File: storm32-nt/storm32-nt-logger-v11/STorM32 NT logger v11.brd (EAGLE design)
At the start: 15.5 x 20 mm, 22 parts, among them IC1 STM32F10XTXU6, IC3 MPU9250, Q1 RESONATORSMD

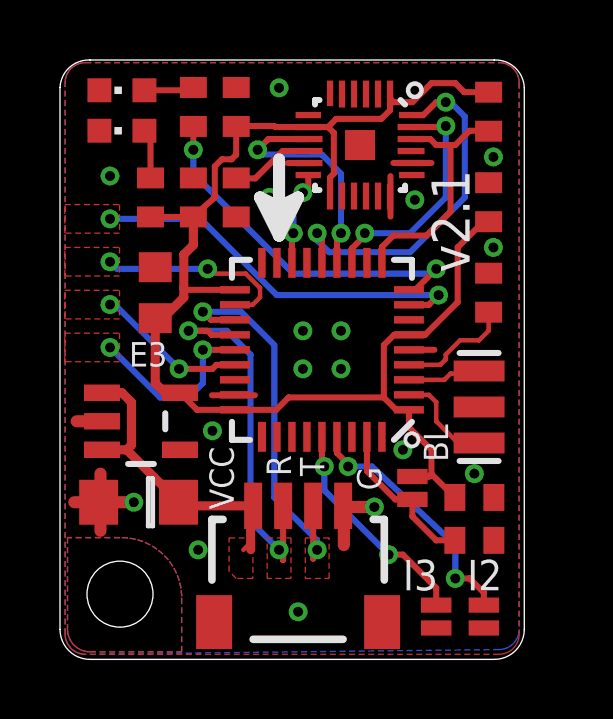
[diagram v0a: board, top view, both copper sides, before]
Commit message: release board v3.3, motor v2.5E, oled, esp
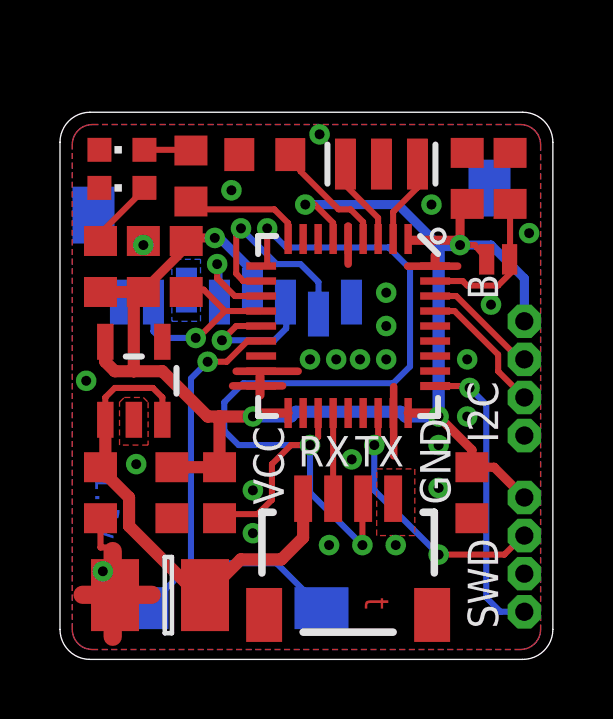
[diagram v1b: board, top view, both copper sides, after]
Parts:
- removed C3, C4, C5, C6: 100n, rcl:C0402
- removed IC1: STM32F10XTXU6, # stm32:VFQFPN36
- removed IC3: MPU9250, # SparkFun2:QFN-24-3X3
- removed NT: NT, con-jst2:SM04B-SRSS-TB
- removed Q1: RESONATORSMD, # SparkFun2:RESONATOR-SMD
- removed R5: 10k, rcl:R0402
- removed SJ1: BOOT0, # SparkFun2:SJ_2S-NO
- removed SJ3: IMU-ID3, # SparkFun2:SJ_2S-NO
- added C10, C11, C9: 100n, rcl:C0603
- added JP1, JP2: SWD, # stdlib:4X1_1P27_OCT_BILEX
- added NTX: NTX, con-jst2:SM04B-SRSS-TB
- added R6: 2.2k, rcl:R0603
- added R7: 10k, rcl:R0603
- added U$1: MICROSD, # adafruit:MICROSD
- added U1: STM32F10XTXU6, # stm32:VFQFPN36
- added Y1: RESONATORSMD, # SparkFun2:RESONATOR-SMD
- C1: device rcl:C0805 -> rcl:SMC_B
- C2: value 1u -> 100n
- C7: value 10n -> 1u; device rcl:C0402 -> rcl:C0603
- C8: device rcl:C0402 -> rcl:C0603
- R1: value 10k -> 4.7k; device rcl:R0402 -> rcl:R0603
- R2: value 4.7k -> 47k; device rcl:R0402 -> rcl:R0603
- R3: value 2.2k -> 47k; device rcl:R0402 -> rcl:R0603
- SJ2: value IMU-ID2 -> BOOT0
- moved R1 15.4 mm to (1.35, 13.1), turned to 90 degrees
- moved C7 13.0 mm to (3.73, 5.56), turned to 270 degrees
- moved R3 12.9 mm to (5.32, 5.56)
- moved SJ2 11.9 mm to (14.6, 13.3), turned to 0 degrees
- moved C2 6.91 mm to (1.35, 5.56), turned to 270 degrees
- moved C1 3.18 mm to (3.33, 2.14)
- moved R2 2.59 mm to (4.21, 13.1)
- moved LED2 1.98 mm to (2.06, 17.0)
- moved LED1 1.90 mm to (2.06, 15.7)
- moved C8 1.72 mm to (6.83, 16.8), turned to 180 degrees
- moved IC2 1.37 mm to (2.46, 9.29), turned to 0 degrees
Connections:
- removed net ADC1: IC1.8
- removed net CANRX: IC1.23
- removed net CANTX: IC1.24
- removed net INT: IC1.16, IC3.12
- removed net N$20: C8.1, IC3.10
- removed net N$4: IC1.32, SJ3.2
- removed net N$7: IC1.33, SJ2.2
- removed net T1CH1: IC1.20
- new net CD1: U$1.CD1, U$1.CD2, U1.15
- new net SCL: JP1.3, U1.33
- new net SDA: JP1.2, U1.34
- net 3.3V: now also C10.1, C11.1, C9.1, JP1.1, JP2.1, R1.1, R2.2, R3.2, SJ2.1, U$1.4, U1.1, U1.19, U1.27, U1.6; no longer C2.1, C4.1, C5.1, C6.1, IC1.1, IC1.19, IC1.27, IC1.6, IC3.1, IC3.13, IC3.8, R2.1, R5.2, SJ1.1
- net 5V: now also C1.+, C2.1, NTX.1; no longer C1.1, NT.1
- net CS: now also U$1.2, U1.11; no longer IC1.10, IC3.22, R5.1
- net GND: now also C1.-, C10.2, C11.2, C9.2, JP1.4, JP2.3, NTX.4, R7.1, U$1.6, U$1.MT1, U$1.MT2, U1.17, U1.18, U1.26, U1.36, U1.5, Y1.2; no longer C1.2, C3.2, C4.2, C5.2, C6.2, IC1.17, IC1.18, IC1.26, IC1.30, IC1.31, IC1.36, IC1.5, IC3.11, IC3.18, IC3.20, NT.4, Q1.2, R1.1, SJ2.1, SJ3.1
- net LED: now also R6.1, U1.9; no longer IC1.9, R3.1
- net N$1: now also C8.1, U1.4; no longer C3.1, IC1.4
- net N$2: now also R6.2; no longer R3.2
- net N$3: now also R7.2, SJ2.2, U1.35; no longer IC1.35, R1.2, SJ1.2
- net N$5: now also U1.2, Y1.1; no longer IC1.2, Q1.1
- net N$6: now also U1.3, Y1.3; no longer IC1.3, Q1.3
- net N$9: now also R1.2; no longer R2.2
- net RX: now also NTX.2, U1.22; no longer IC1.22, NT.2
- net SCK: now also U$1.5, U1.12; no longer IC1.12, IC3.23
- net SDI: now also U$1.3, U1.14; no longer IC1.14, IC3.24
- net SDO: now also R2.1, U$1.7, U1.13; no longer IC1.13, IC3.9
- net SWCLK: now also JP2.4, U1.28; no longer IC1.28
- net SWDIO: now also JP2.2, U1.25; no longer IC1.25
- net TX: now also NTX.3, R3.1, U1.10, U1.21; no longer IC1.21, NT.3
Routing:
- net TX: track 13.5 -> 32.3 mm, vias 2 -> 3
- net CD1: track 0.00 -> 17.0 mm, vias 0 -> 1
- net ADC1: track 13.1 -> 0.00 mm, vias 2 -> 0
- net RX: track 13.1 -> 3.09 mm, vias 2 -> 0
- net SWCLK: track 0.00 -> 9.85 mm, vias 0 -> 1
- net SWDIO: track 0.00 -> 8.78 mm, vias 0 -> 2
- net N$7: track 8.43 -> 0.00 mm, vias 2 -> 0
- net LED: track 12.3 -> 4.11 mm, vias 2 -> 0
- net N$4: track 7.47 -> 0.00 mm, vias 2 -> 0
- net SDI: track 12.0 -> 4.70 mm, vias 2 -> 1
- net 3.3V: track 47.1 -> 54.3 mm, vias 0 -> 5
- net T1CH1: track 6.62 -> 0.00 mm, vias 2 -> 0
- net CANRX: track 6.16 -> 0.00 mm, vias 2 -> 0
- net 5V: track 11.5 -> 17.0 mm
- net CANTX: track 5.11 -> 0.00 mm, vias 2 -> 0
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- removed copper zone on layer 1, net 5V
- removed copper zone on layer 1, net ADC1
- removed copper zone on layer 1, net CANRX
- removed copper zone on layer 1, net CANTX
- removed copper zone on layer 1, net RX
- removed copper zone on layer 1, net T1CH1
- removed copper zone on layer 1, net TX
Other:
- board size 15.5 x 20 mm -> 16.4 x 18.2 mm
- board text added: "B"
- board text added: "I2C"
- board text added: "SWD"
- board text added: "t"
- board text added: "v1.1"
- board text added: "www.olliw.eu NT Logger v1.1"
- board text removed: "ADC1 EXT0"
- board text removed: "BL"
- board text removed: "CANRX EXT3"
- board text removed: "CANTX EXT2"
- board text removed: "E3"
- board text removed: "G"
- board text removed: "I2"
- board text removed: "I3"
- board text removed: "NT IMU mpu9250"
- board text removed: "R"
- board text removed: "T"
- board text removed: "T1CH1 EXT1"
- board text removed: "v2.1"
- board text removed: "www.olliw.eu"
